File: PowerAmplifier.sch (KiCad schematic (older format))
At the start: 36 parts, among them K1 INPUT, K2 OUTPUT, P1 POWER

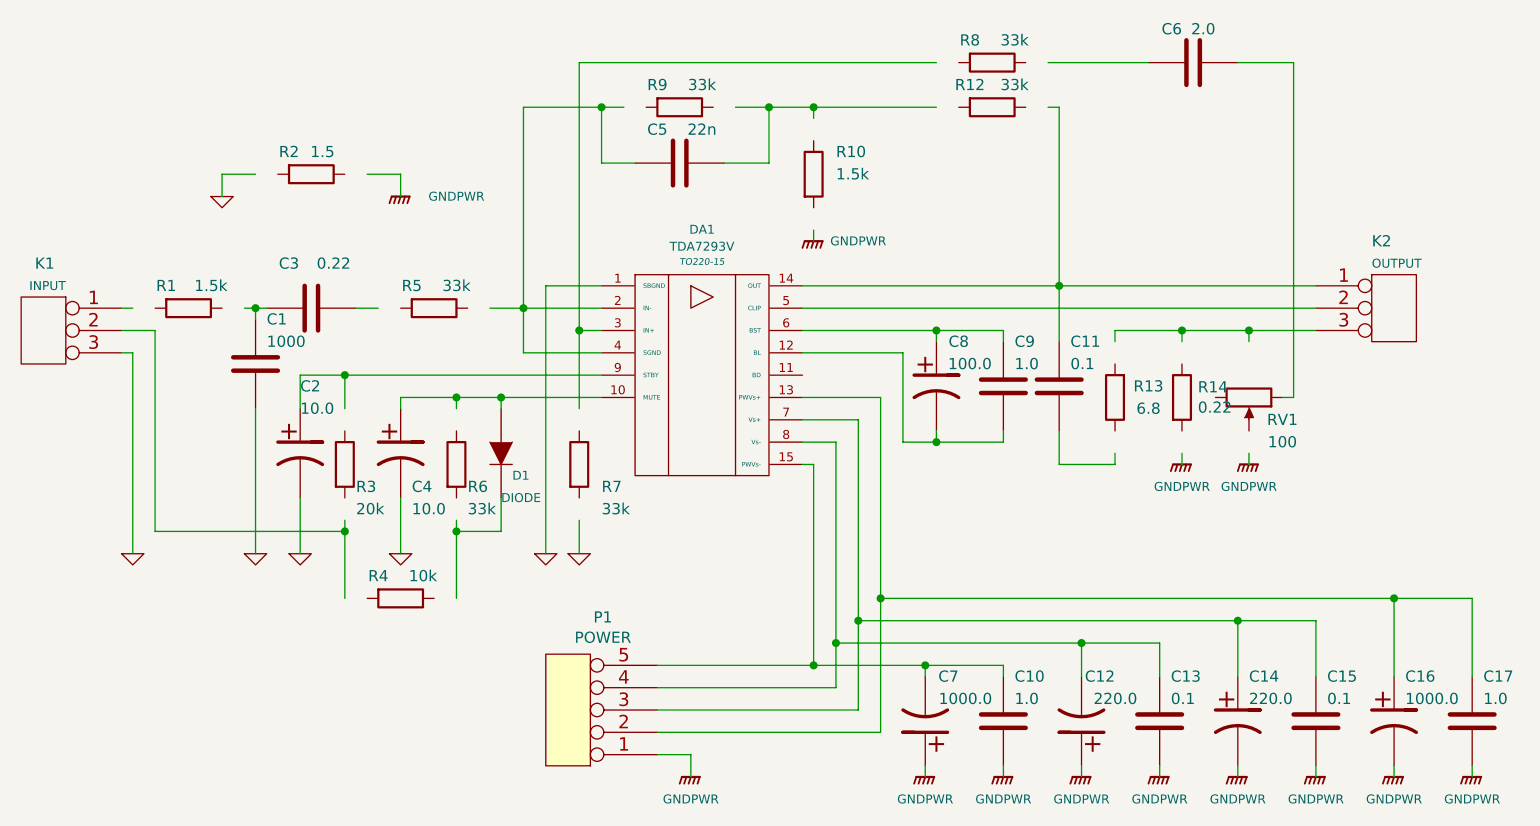
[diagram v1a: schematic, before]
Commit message: Add power
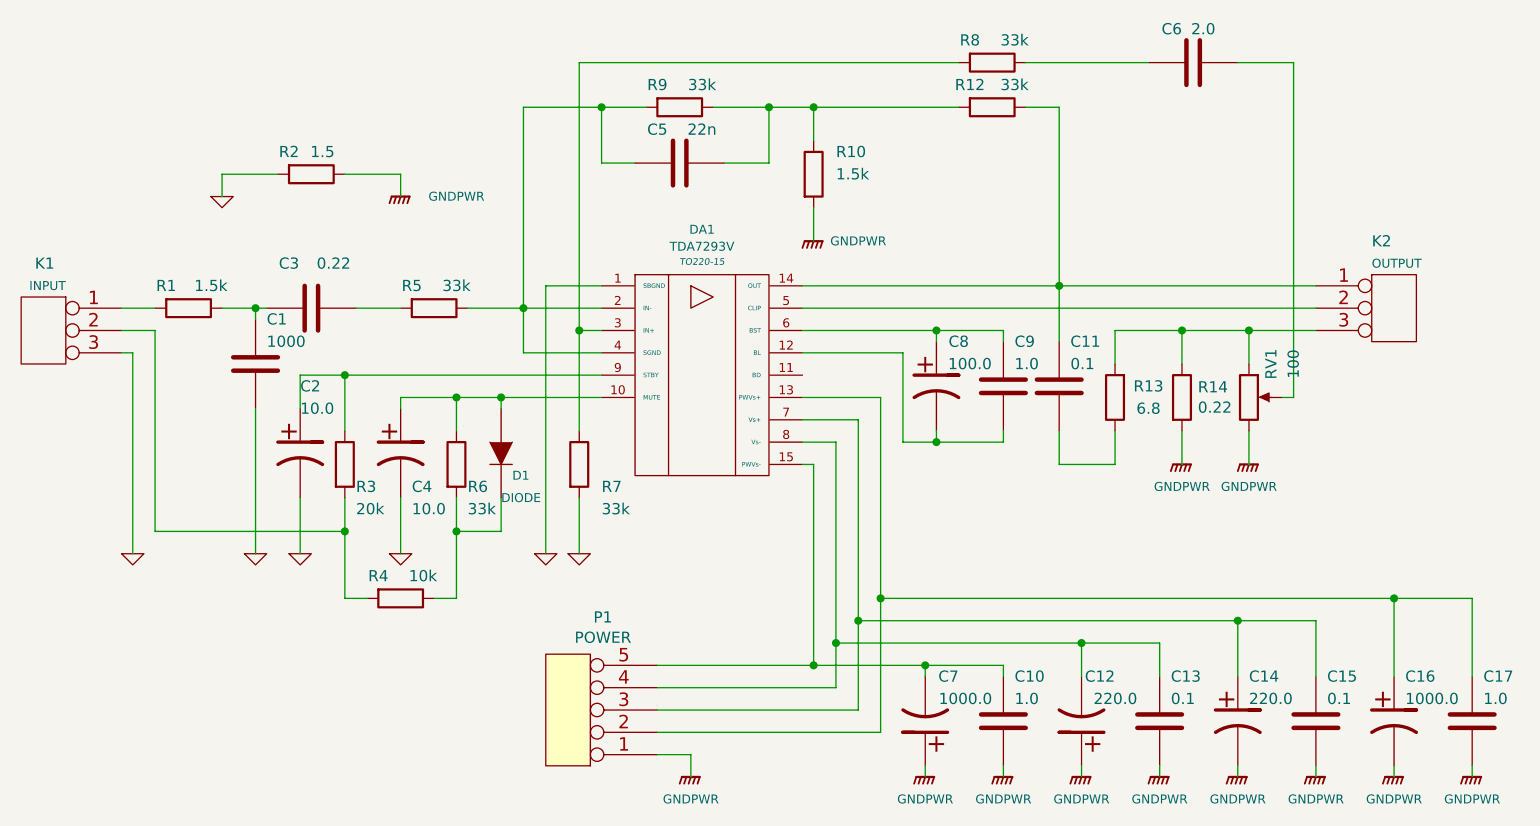
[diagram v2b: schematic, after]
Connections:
- wire segments 102 -> 104
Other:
- moved on the sheet: RV1
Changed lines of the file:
@@
 EESchema Schematic File Version 2
 LIBS:amplifier-rescue
-LIBS:power
-LIBS:device
-LIBS:transistors
-LIBS:conn
-LIBS:linear
-LIBS:regul
-LIBS:74xx
-LIBS:cmos4000
-LIBS:adc-dac
-LIBS:memory
-LIBS:xilinx
-LIBS:microcontrollers
-LIBS:dsp
-LIBS:microchip
-LIBS:analog_switches
-LIBS:motorola
-LIBS:texas
-LIBS:intel
-LIBS:audio
-LIBS:interface
-LIBS:digital-audio
-LIBS:philips
-LIBS:display
-LIBS:cypress
-LIBS:siliconi
-LIBS:opto
-LIBS:atmel
-LIBS:contrib
-LIBS:valves
-LIBS:tda7293v
-LIBS:ad1955
-LIBS:src4392i
-LIBS:cdclvc1104
 LIBS:amplifier-cache
-EELAYER 26 0
+EELAYER 25 0
 EELAYER END
 $Descr A4 11693 8268
@@
 F 3 "" H 6300 2300 60  0001 C CNN
 	1    6300 2300
-	0    1    1    0
+	1    0    0    -1
 $EndComp
 $Comp
@@
 	5700 2000 6600 2000
 Wire Wire Line
-	3050 1000 3500 1000
+	3050 1000 3600 1000
 Wire Wire Line
 	3050 1000 3050 2100
 Wire Wire Line
-	2900 1900 3400 1900
-Wire Wire Line
-	2300 1900 2400 1900
+	2800 1900 3400 1900
+Wire Wire Line
+	2300 1900 2500 1900
 Connection ~ 3050 1900
 Wire Wire Line
@@
 	3950 1250 4150 1250
 Wire Wire Line
-	4350 1000 4350 1050
+	4350 1000 4350 1150
 Connection ~ 4350 1000
 Wire Wire Line
@@
 Connection ~ 3400 1000
 Wire Wire Line
-	4350 1550 4350 1600
+	4350 1450 4350 1600
 Connection ~ 6000 2000
 Wire Wire Line
-	1800 1900 1900 1900
+	1700 1900 1900 1900
 Wire Wire Line
 	1850 1950 1850 1900
@@
 	5450 2600 5700 2600
 Wire Wire Line
-	5700 2600 5700 2550
-Wire Wire Line
-	5700 2050 5700 2000
-Wire Wire Line
-	6000 2550 6000 2600
+	5700 2600 5700 2450
+Wire Wire Line
+	5700 2000 5700 2150
 Wire Wire Line
 	5200 2500 5200 2450
@@
 Connection ~ 4900 2500
 Wire Wire Line
-	2350 1300 2500 1300
+	2250 1300 2500 1300
 Wire Wire Line
 	2500 1300 2500 1400
 Wire Wire Line
-	1850 1300 1700 1300
+	1700 1300 1950 1300
 Wire Wire Line
 	1700 1300 1700 1400
@@
 	2500 2300 3400 2300
 Wire Wire Line
-	2750 2300 2750 2350
+	2750 2300 2750 2450
 Wire Wire Line
 	2500 2350 2500 2300
@@
 	2050 2200 2050 2350
 Wire Wire Line
-	2250 2350 2250 2200
+	2250 2200 2250 2450
 Connection ~ 2250 2200
 Wire Wire Line
@@
 	2950 2900 2750 2900
 Wire Wire Line
-	2750 2850 2750 3200
+	2750 2750 2750 3200
 Wire Wire Line
 	2500 2750 2500 3000
@@
 Connection ~ 2750 2900
 Wire Wire Line
-	2250 2850 2250 3200
+	2250 2750 2250 3200
 Wire Wire Line
 	1400 2900 2250 2900
@@
 	4300 1900 6600 1900
 Wire Wire Line
-	1250 1900 1300 1900
+	1250 1900 1400 1900
 Wire Wire Line
 	1300 2100 1300 3000
@@
 $EndComp
 Wire Wire Line
-	4000 1000 4900 1000
+	3900 1000 5000 1000
 $Comp
 L C-RESCUE-amplifier C3
@@
 $EndComp
 Wire Wire Line
-	3300 2850 3300 3000
-Wire Wire Line
-	3300 800  3300 2350
+	3300 2750 3300 3000
+Wire Wire Line
+	3300 800  3300 2450
 Wire Wire Line
 	3300 2000 3400 2000
@@
 Connection ~ 5450 1800
 Wire Wire Line
-	5400 1000 5450 1000
+	5300 1000 5450 1000
 Connection ~ 3300 2000
 $Comp
@@
 $EndComp
 Wire Wire Line
-	4900 800  3300 800
+	3300 800  5000 800
 $Comp
 L GNDPWR #PWR020
@@
 $EndComp
 Wire Wire Line
-	6300 2550 6300 2600
-Wire Wire Line
-	6300 2050 6300 2000
+	6300 2000 6300 2150
 Connection ~ 6300 2000
 Wire Wire Line
-	6000 2050 6000 2000
+	6000 2000 6000 2150
 Wire Wire Line
 	6500 800  6500 2300
@@
 	3400 1800 3150 1800
 Wire Wire Line
-	5400 800  5850 800
+	5300 800  5850 800
+Wire Wire Line
+	2250 3200 2350 3200
+Wire Wire Line
+	2750 3200 2650 3200
+Wire Wire Line
+	6300 2450 6300 2600
+Wire Wire Line
+	6000 2450 6000 2600
 $EndSCHEMATC
